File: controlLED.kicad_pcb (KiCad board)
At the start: 2 copper layers, 135.9 x 74.9 mm, 47 parts, among them CON1 BARREL_JACK, J1 connector, J2 connector, J3 connector, J4 connector, J5 connector, J6 connector, J7 connector, J8 connector, J9 connector, P1 CONN_A0-1, P10 CONN_01X06, P11 CONN_01X02, P3 ESP32_sparkfun, P5 CONN_D0-1, P6 CONN_A0-1, P7 CONN_D0-1, P8 CONN_UART, P9 CONN_I2C, U1 LD1117S50TR, U2 LD1117S33TR

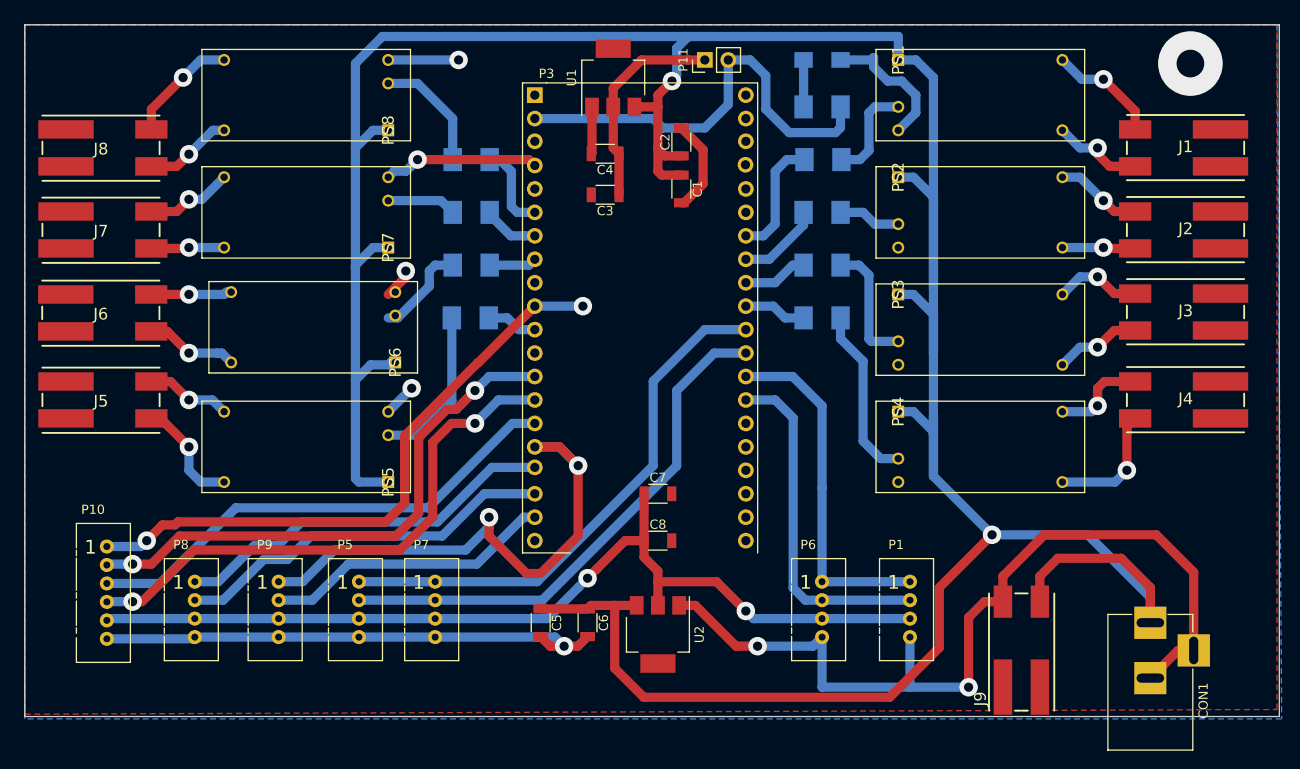
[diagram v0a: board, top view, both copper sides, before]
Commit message: version1.0
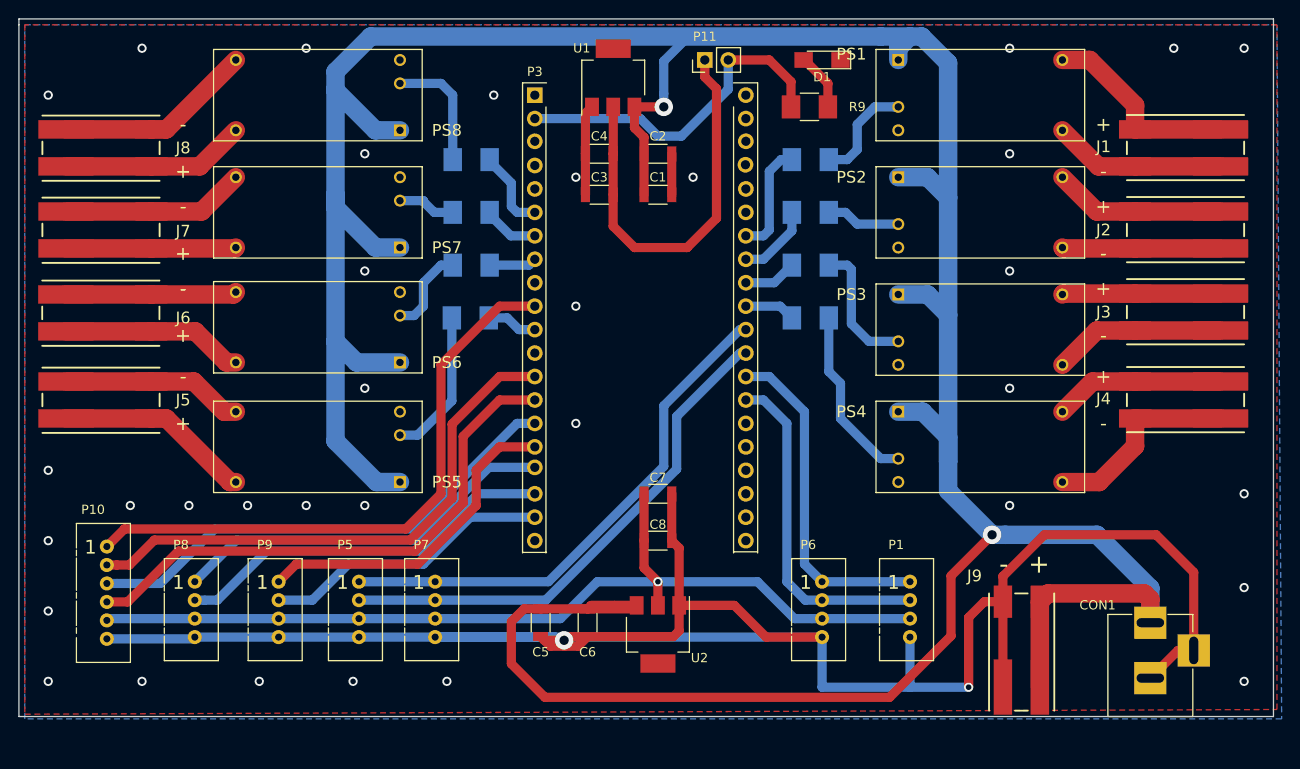
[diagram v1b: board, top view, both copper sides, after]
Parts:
- D1, R9: moved to F.Cu
- moved C2 2.84 mm to (147.3, 64.8), turned to 0 degrees
- moved C1 2.62 mm to (147.3, 69.2), turned to 0 degrees
- moved R1 1.36 mm to (163.8, 65.4)
- moved R9 1.36 mm to (163.7, 59.7), turned to 180 degrees
- moved PS5 1.27 mm to (119.4, 100.3)
- moved PS7 1.27 mm to (119.4, 74.9)
- moved PS8 1.27 mm to (119.4, 62.2)
- moved R2 1.27 mm to (163.8, 71.1)
- moved R3 1.27 mm to (163.8, 76.8)
- moved R4 1.27 mm to (163.8, 82.5)
- moved C3 0.63 mm to (141.0, 69.2)
- moved C4 0.63 mm to (141.0, 64.8)
- moved PS6 0.51 mm to (119.4, 87.4)
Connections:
- J1 pad 2: (no net) -> Net-(J1-Pad1)
- J1 pad 4: (no net) -> Net-(J1-Pad3)
- J2 pad 2: (no net) -> Net-(J2-Pad1)
- J2 pad 4: (no net) -> Net-(J2-Pad3)
- J3 pad 2: (no net) -> Net-(J3-Pad1)
- J3 pad 4: (no net) -> Net-(J3-Pad3)
- J4 pad 2: (no net) -> Net-(J4-Pad1)
- J4 pad 4: (no net) -> Net-(J4-Pad3)
- J5 pad 2: (no net) -> Net-(J5-Pad1)
- J5 pad 4: (no net) -> Net-(J5-Pad3)
- J6 pad 2: (no net) -> Net-(J6-Pad1)
- J6 pad 4: (no net) -> Net-(J6-Pad3)
- J7 pad 2: (no net) -> Net-(J7-Pad1)
- J7 pad 4: (no net) -> Net-(J7-Pad3)
- J8 pad 2: (no net) -> Net-(J8-Pad1)
- J8 pad 4: (no net) -> Net-(J8-Pad3)
- J9 pad 2: (no net) -> /VCC24
- J9 pad 4: (no net) -> GND
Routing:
- net /VCC24: track 355.3 -> 406.7 mm
- net GND: track 215.7 -> 249.1 mm, vias 7 -> 36
- net /SCL: track 60.0 -> 36.0 mm, vias 2 -> 0
- net Net-(C3-Pad1): track 23.0 -> 44.1 mm
- net Net-(J7-Pad1): track 7.92 -> 18.4 mm, vias 1 -> 0
- net Net-(J8-Pad1): track 9.49 -> 20.0 mm, vias 1 -> 0
- net Net-(J5-Pad3): track 9.23 -> 19.8 mm, vias 1 -> 0
- net Net-(J7-Pad3): track 9.42 -> 19.9 mm, vias 1 -> 0
- net Net-(P11-Pad2): track 47.3 -> 37.5 mm
- net Net-(J6-Pad3): track 8.76 -> 18.5 mm, vias 1 -> 0
- net Net-(J6-Pad1): track 10.1 -> 19.8 mm, vias 1 -> 0
- net Net-(J1-Pad1): track 12.2 -> 21.8 mm, vias 1 -> 0
- net Net-(J2-Pad3): track 7.92 -> 17.2 mm, vias 1 -> 0
- net Net-(J3-Pad3): track 9.42 -> 18.7 mm, vias 1 -> 0
- net Net-(J2-Pad1): track 9.42 -> 18.7 mm, vias 1 -> 0
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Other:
- board size 135.9 x 74.9 mm -> 135.9 x 75.6 mm
- board text added: "+"
- board text added: "-"
